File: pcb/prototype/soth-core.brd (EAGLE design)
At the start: 100 x 80 mm, 22 parts, among them IC1 AE-FT231X(FT231X) USB-Serial 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, IC2 REG1117, IC3 TC7SZ125F, IC4 TC7SZ125F, IC5 12113(LPS331AP) Pressure Sens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, U1 ATXMEGA32D4-AU, X1 5V/4A

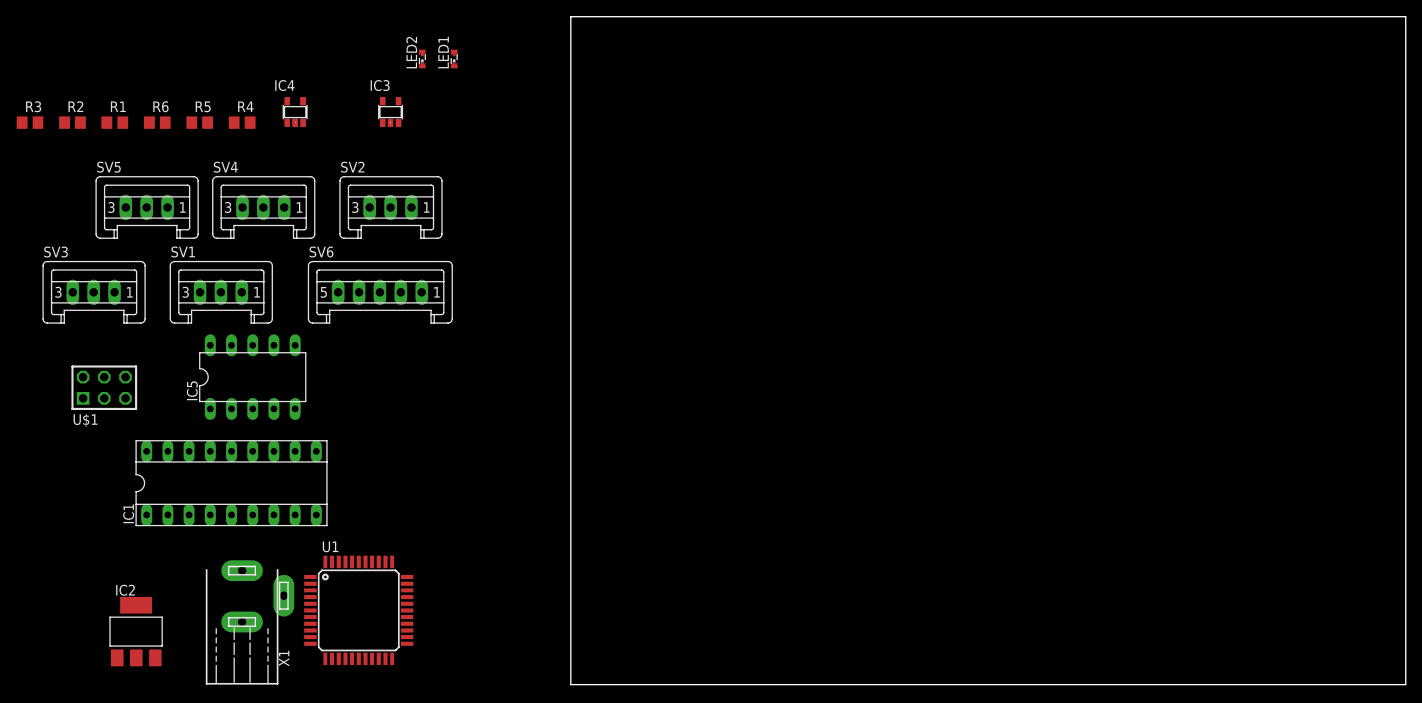
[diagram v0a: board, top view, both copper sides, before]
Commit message: Created v0.1
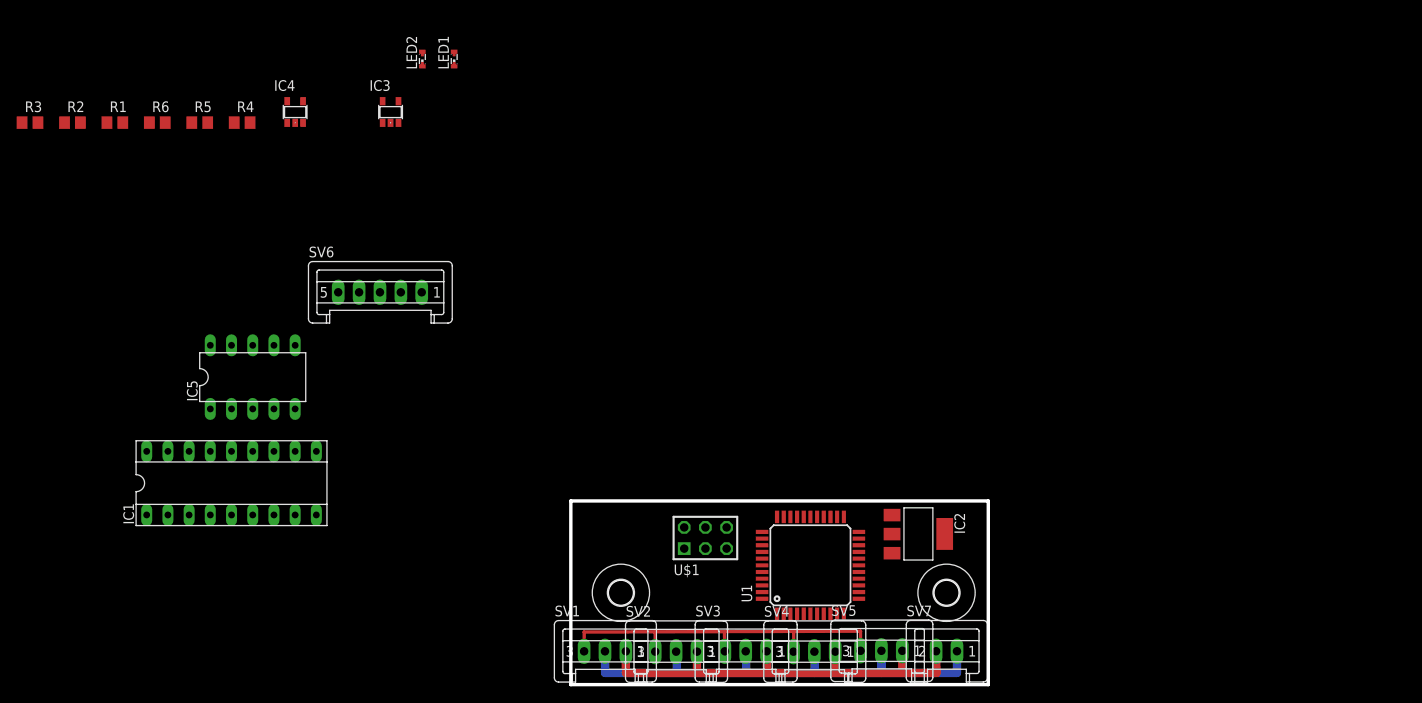
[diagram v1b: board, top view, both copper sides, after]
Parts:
- removed X1: 5V/4A, con-conrad:733980-62
- added H1, H2: MOUNT-HOLE3.0, holes:3,0
- added SV7: PowerSupply, con-amp-mt:S02P
- moved SV5 102.8 mm to (37.2, 4.05)
- moved IC2 94.4 mm to (41.6, 18.1), turned to 270 degrees
- moved SV3 89.2 mm to (20.9, 3.99)
- moved SV4 84.8 mm to (29.2, 3.95)
- moved U$1 74.2 mm to (16.1, 17.6)
- moved SV2 63.2 mm to (12.6, 3.95)
- moved SV1 63.0 mm to (4.09, 3.99)
- moved U1 54.4 mm to (28.7, 14.3), turned to 90 degrees
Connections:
- removed net N$16: IC5.10, IC5.9
- net +3V3: now also IC5.10, IC5.5, IC5.9
- net +5V: now also SV7.1; no longer X1.2, X1.3
- net GND: now also IC5.4, SV7.2; no longer X1.1
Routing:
- net +5V: track 0.00 -> 65.4 mm
- net GND: track 0.00 -> 52.7 mm
- net N$1: track 0.00 -> 44.9 mm
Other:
- board size 100 x 80 mm -> 50 x 22 mm
